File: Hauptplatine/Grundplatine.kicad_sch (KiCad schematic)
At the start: 8 parts, among them IC12 Arduino_Nano_v2.x, IC26 74HC00

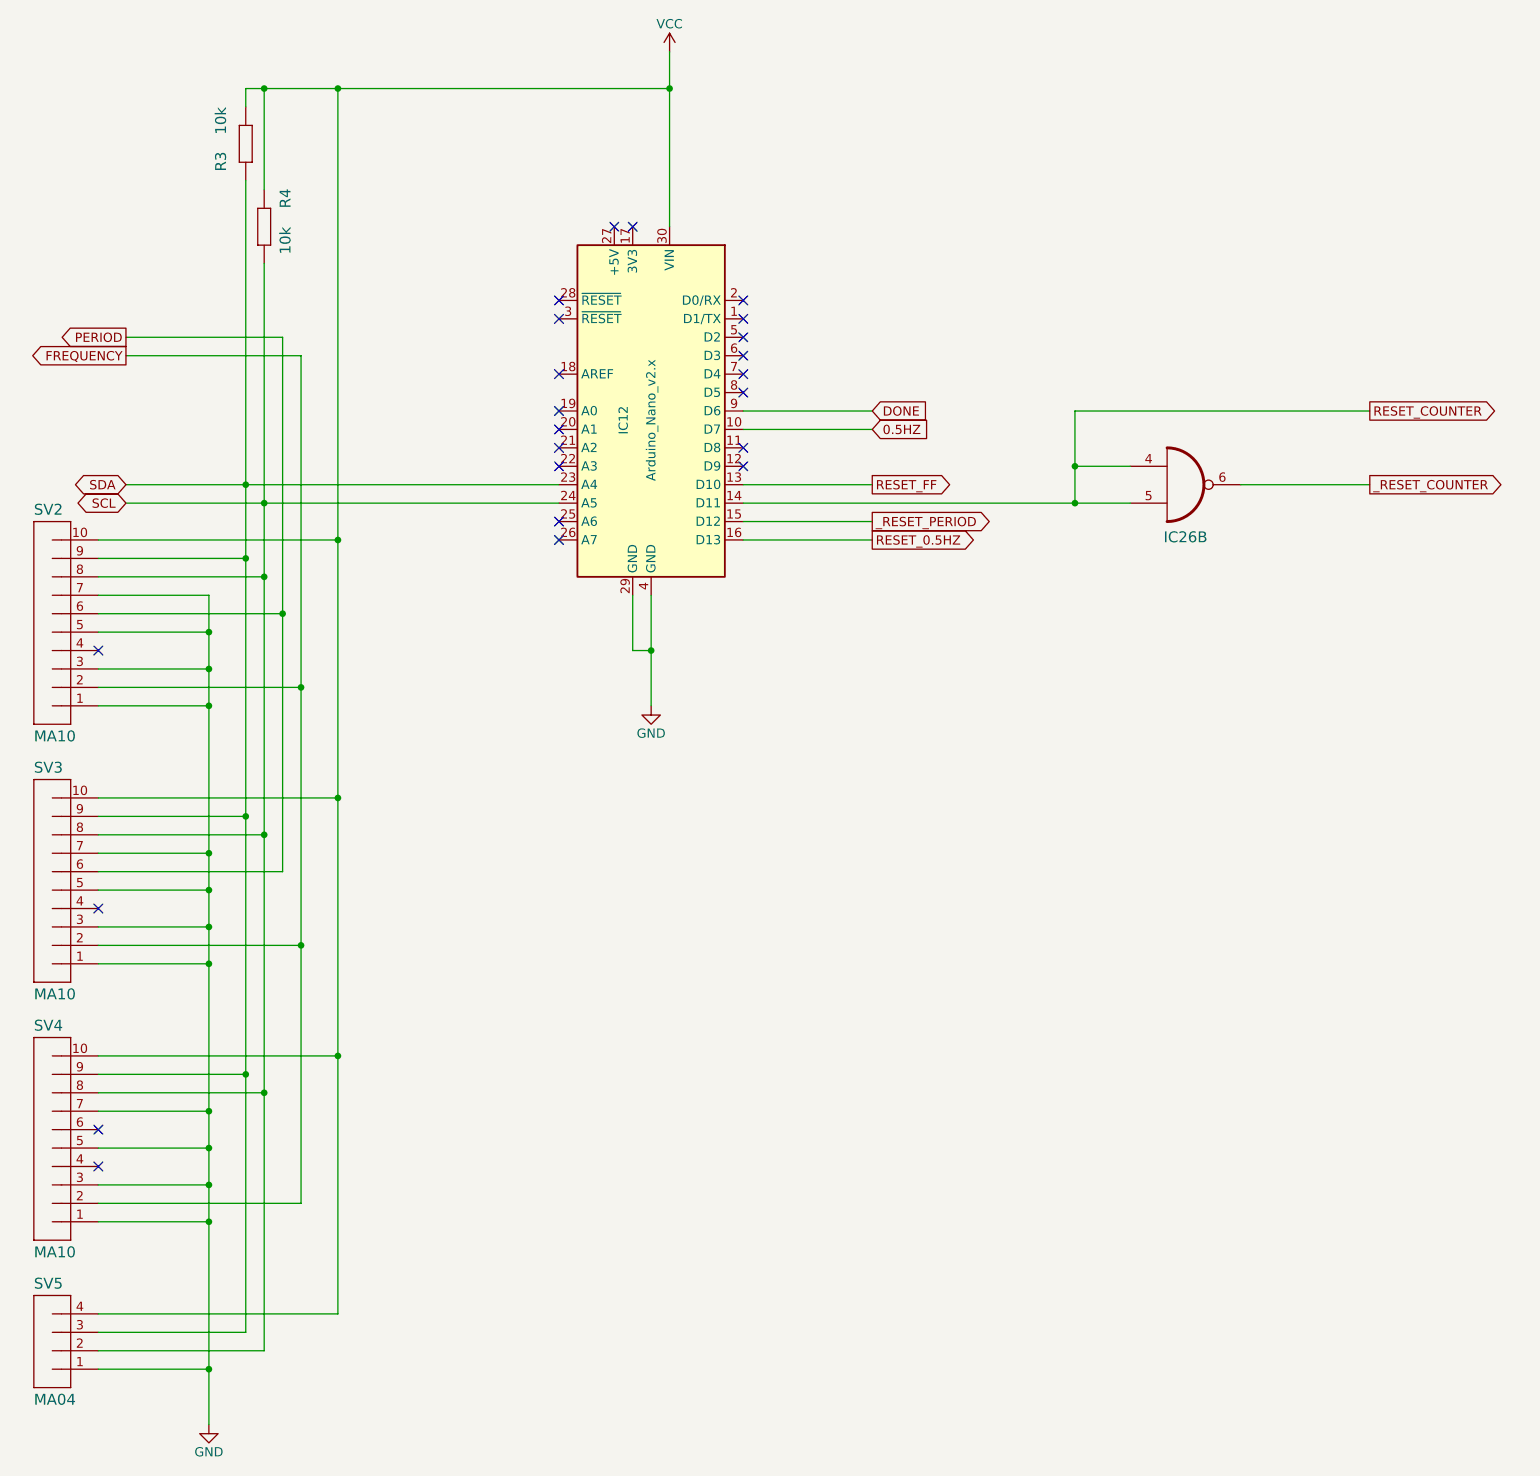
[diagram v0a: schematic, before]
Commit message: Update
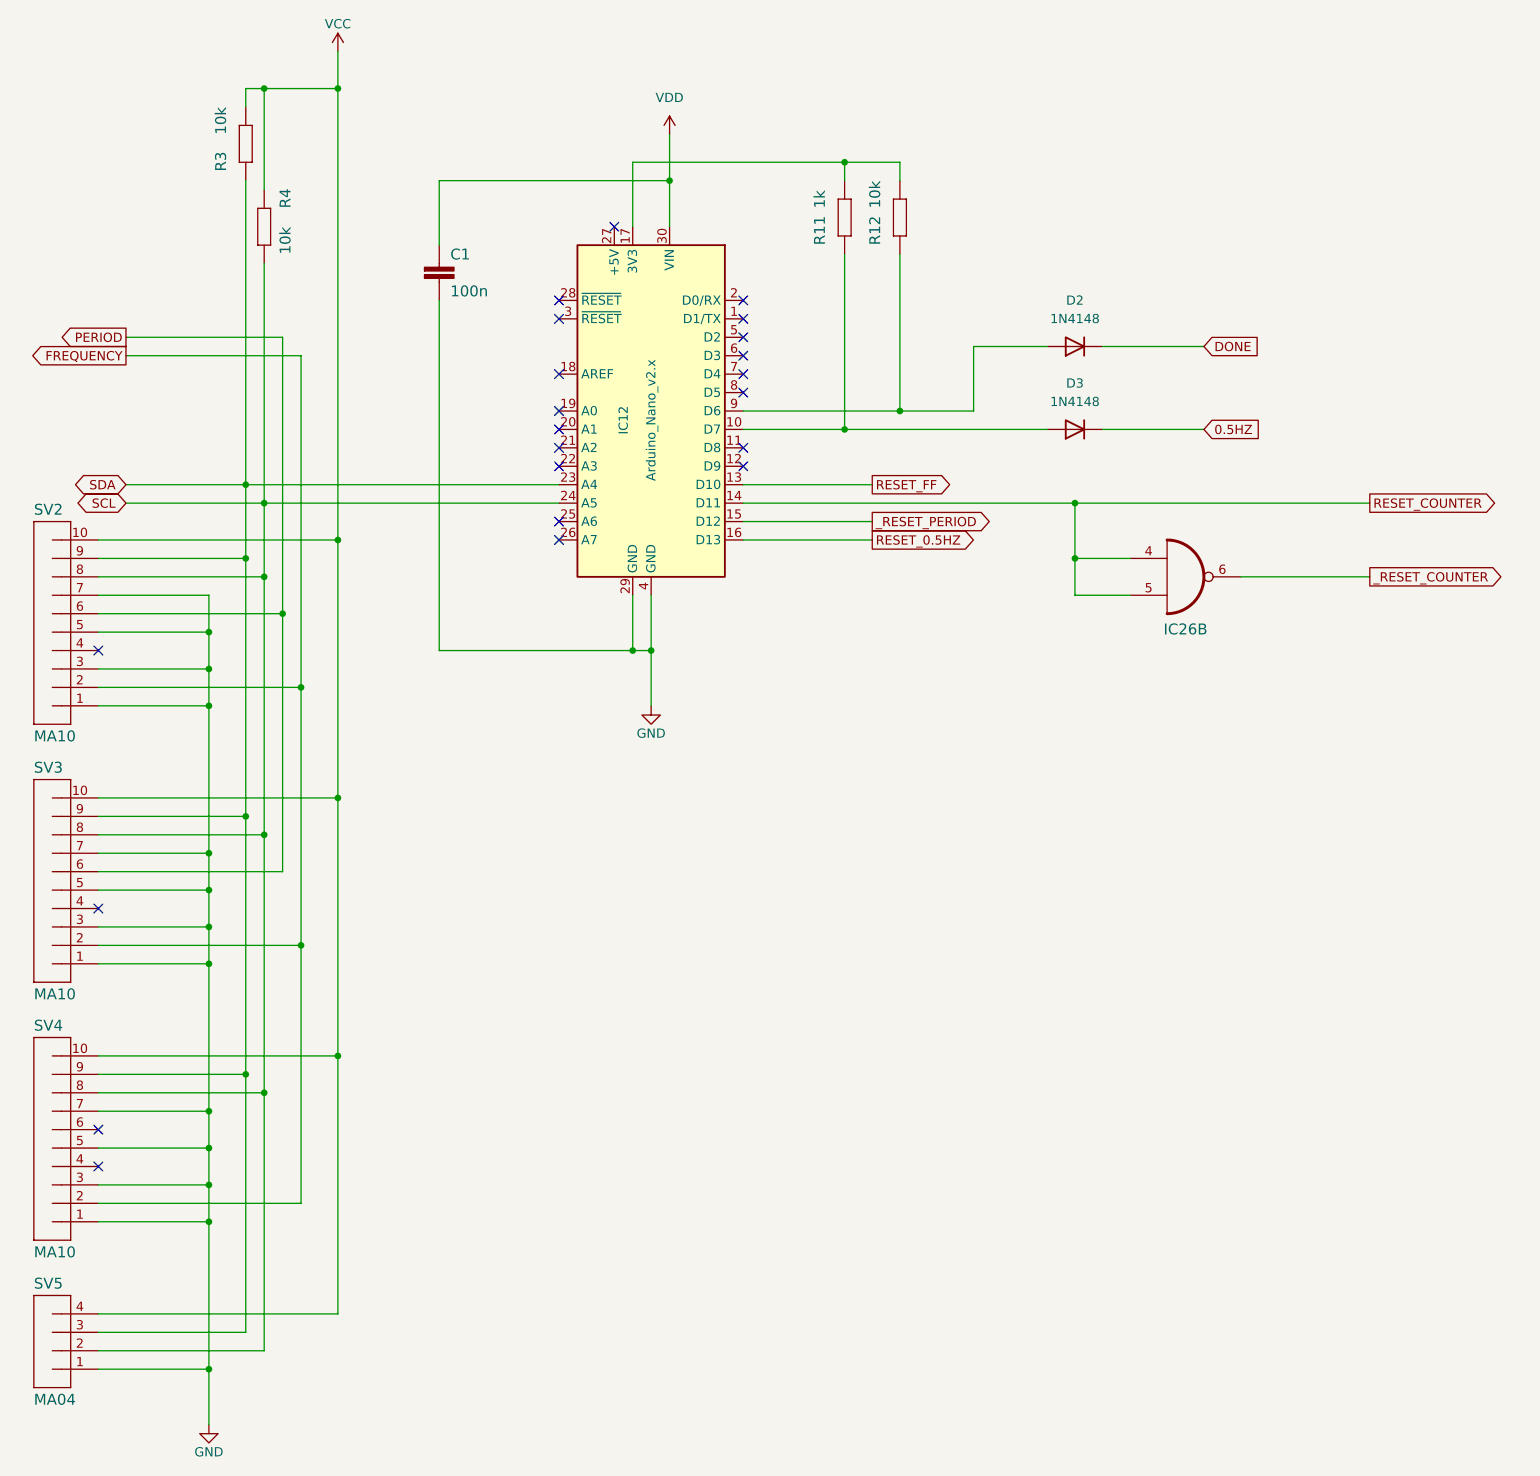
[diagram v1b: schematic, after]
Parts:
- added C1: 100n, Capacitor_THT:C_Rect_L10.0mm_W4.0mm_P7.50mm_FKS3_FKP3, symbol Hauptplatine-rescue:C-EUC0603-Zähler-eagle-import
- added D2, D3: 1N4148, Diode_THT:D_DO-35_SOD27_P7.62mm_Horizontal, symbol Device:D
- added R11: 1k, Resistor_THT:R_Axial_DIN0204_L3.6mm_D1.6mm_P1.90mm_Vertical, symbol Hauptplatine-rescue:R-EU_M0805-Grundplatine-eagle-import
- added R12: 10k, Resistor_THT:R_Axial_DIN0204_L3.6mm_D1.6mm_P1.90mm_Vertical, symbol Hauptplatine-rescue:R-EU_M0805-Grundplatine-eagle-import
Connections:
- net 0.5HZ: now also D3.1 (K); no longer IC12.10 (D7)
- net DONE: now also D2.1 (K); no longer IC12.9 (D6)
- net GND: now also C1.2
- net VCC: no longer IC12.30 (VIN)
- net at IC12.17 (3V3): now also R11.2, R12.2
- new net: D3.2 (A), IC12.10 (D7), R11.1
- new net: D2.2 (A), IC12.9 (D6), R12.1
- new net VDD: C1.1, IC12.30 (VIN)
- no-connect marks 23 -> 22
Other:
- moved on the sheet: IC26B
